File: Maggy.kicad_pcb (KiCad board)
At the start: 2 copper layers, 160 x 100 mm, 75 parts, among them CN1 0430450800, CN2 430451000, J1 XY308-2.54-2P, J2 XY308-2.54-2P, J3 XY308-2.54-2P, J4 XY308-2.54-2P, U1 CH224K, U10 INA214AIDCKR, U11 Socket for Teensy 4.1 (2x 1x2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, U12 INA214AIDCKR, U13 INA214AIDCKR, U14 TMAG5170A2DGKR, U15 TMAG5170A2DGKR, U16 TMAG5170A2DGKR, U17 TMAG5170A2DGKR, U18 TMAG5170A2DGKR, U2 A4950ELJTR-T, U3 A4950ELJTR-T, U4 A4950ELJTR-T, U5 A4950ELJTR-T, U6 TLV2372, U7 LM1117S-3.3, U8 LM1117S-5.0, U9 INA214AIDCKR

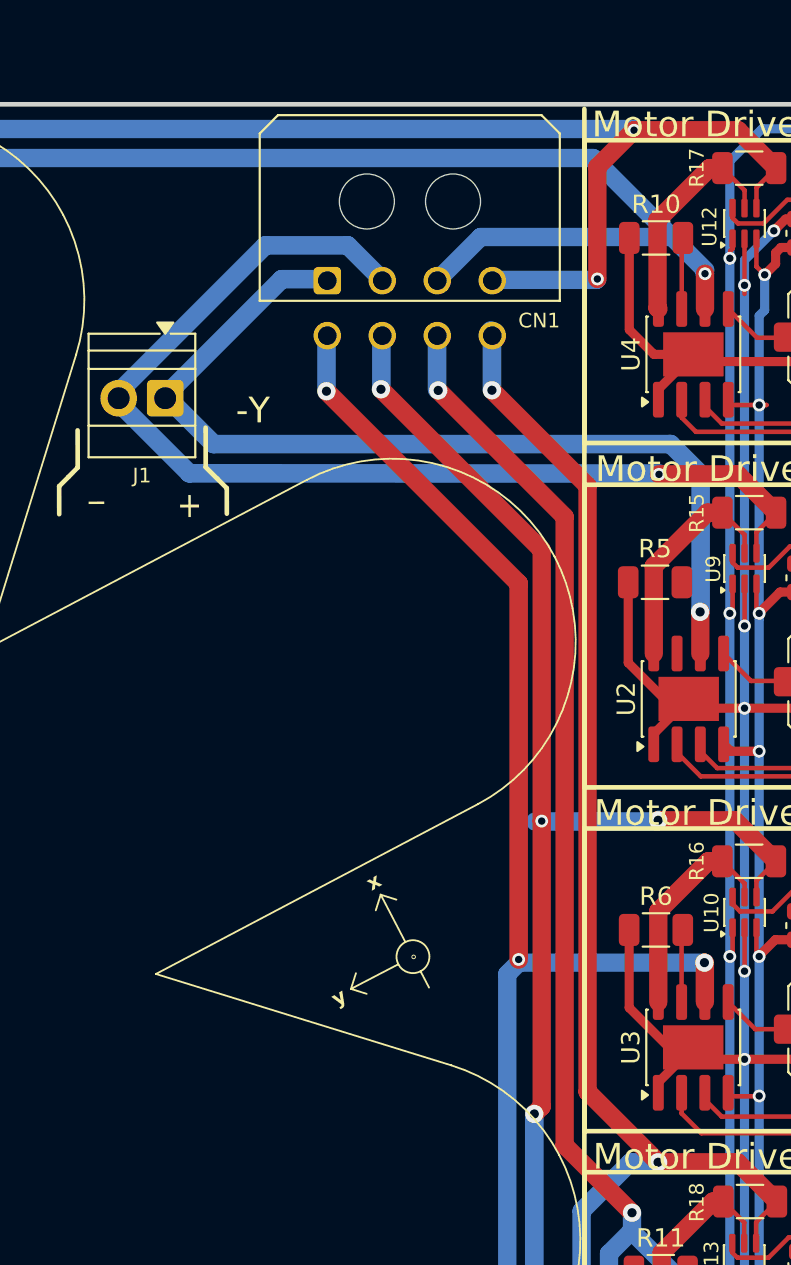
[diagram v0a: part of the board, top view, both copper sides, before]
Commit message: fix: routing for CN1
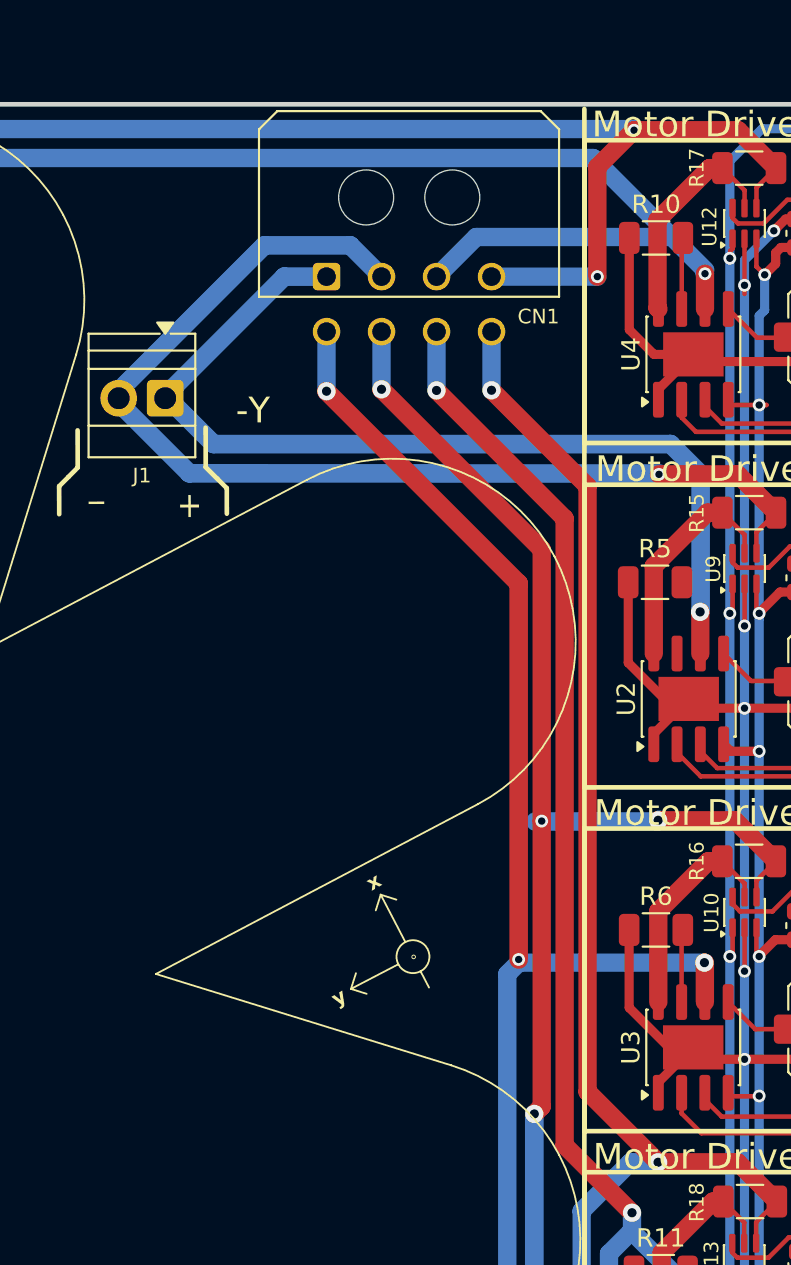
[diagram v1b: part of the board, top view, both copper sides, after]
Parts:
- moved CN1 0.22 mm to (155.4, 69.4)
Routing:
- net 4_1: track 94.3 -> 94.9 mm
